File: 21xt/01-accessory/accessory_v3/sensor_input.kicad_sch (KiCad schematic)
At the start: 3 parts, among them J1 Conn_02x23_Counter_Clockwise, J2 Mezzanine Edge

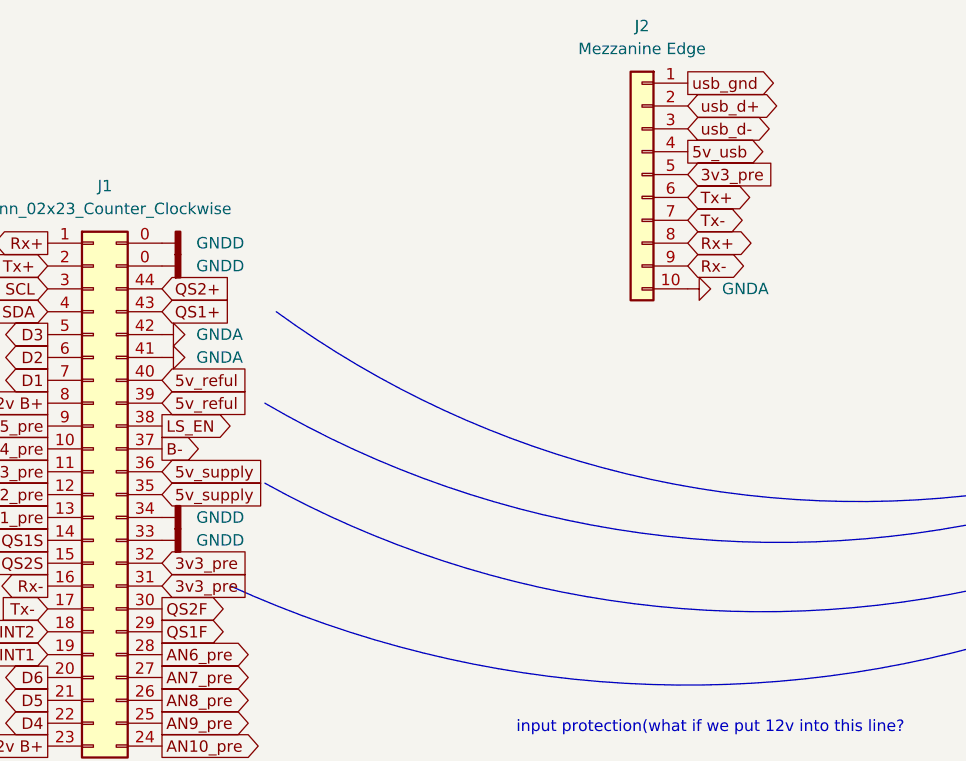
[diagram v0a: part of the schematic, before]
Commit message: prod
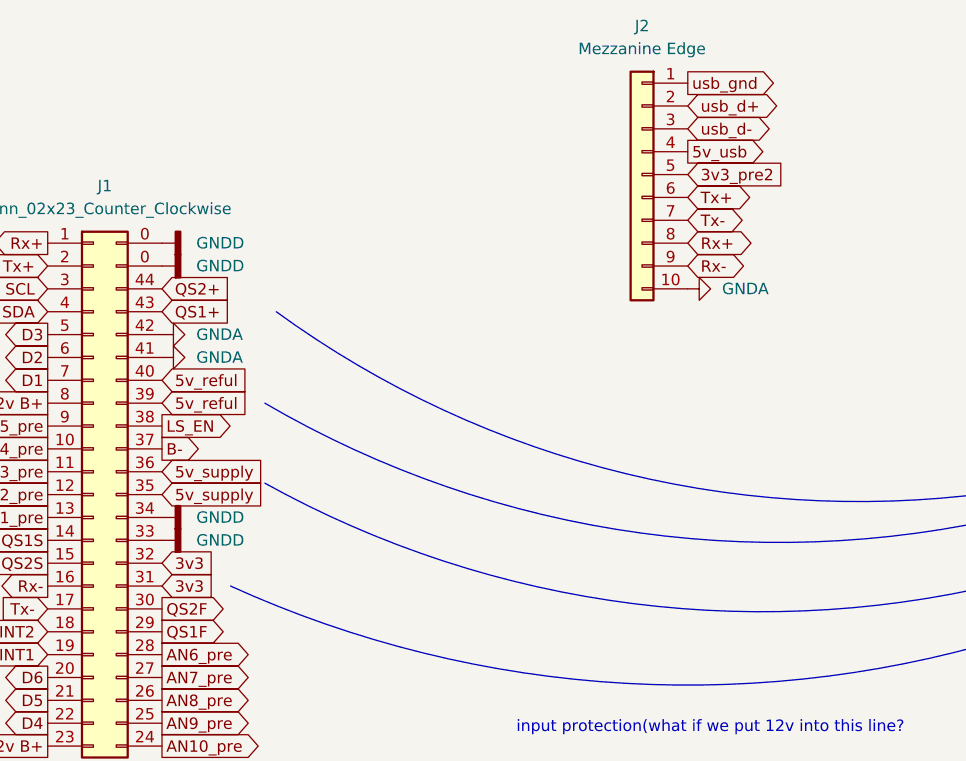
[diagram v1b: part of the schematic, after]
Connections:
- net 3v3_pre renamed 3v3
- net 3v3: no longer J2.5 (Pin_5)
- new net 3v3_pre2: J2.5 (Pin_5)
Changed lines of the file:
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@@
+		)
+	)
+	(global_label "3v3"
+		(shape input)
+		(at 139.7 102.87 0)
+		(fields_autoplaced yes)
+		(effects
+			(font
+				(size 1.27 1.27)
+			)
+			(justify left)
+		)
+		(property "Intersheetrefs" "${INTERSHEET_REFS}"
+			(at 146.0718 102.87 0)
+			(effects
+				(font
+					(size 1.27 1.27)
+				)
+				(justify left)
+				(hide yes)
+			)
 		)
 	)
@@
 		)
 	)
-	(global_label "3v3_pre"
-		(shape input)
-		(at 139.7 102.87 0)
-		(fields_autoplaced yes)
-		(effects
-			(font
-				(size 1.27 1.27)
-			)
-			(justify left)
-		)
-		(property "Intersheetrefs" "${INTERSHEET_REFS}"
-			(at 150.0632 102.87 0)
-			(effects
-				(font
-					(size 1.27 1.27)
-				)
-				(justify left)
-				(hide yes)
-			)
-		)
-	)
 	(global_label "12v B+"
 		(shape output)
@@
 		)
 	)
+	(global_label "3v3_pre2"
+		(shape input)
+		(at 198.12 59.69 0)
+		(fields_autoplaced yes)
+		(effects
+			(font
+				(size 1.27 1.27)
+			)
+			(justify left)
+		)
+		(property "Intersheetrefs" "${INTERSHEET_REFS}"
+			(at 209.6927 59.69 0)
+			(effects
+				(font
+					(size 1.27 1.27)
+				)
+				(justify left)
+				(hide yes)
+			)
+		)
+	)
 	(global_label "GPIO{slash}INT2"
 		(shape bidirectional)
@@
 		)
 	)
+	(global_label "3v3"
+		(shape input)
+		(at 139.7 105.41 0)
+		(fields_autoplaced yes)
+		(effects
+			(font
+				(size 1.27 1.27)
+			)
+			(justify left)
+		)
+		(property "Intersheetrefs" "${INTERSHEET_REFS}"
+			(at 146.0718 105.41 0)
+			(effects
+				(font
+					(size 1.27 1.27)
+				)
+				(justify left)
+				(hide yes)
+			)
+		)
+	)
 	(global_label "AN7_pre"
 		(shape output)
@@
 		)
 	)
-	(global_label "3v3_pre"
-		(shape input)
-		(at 139.7 105.41 0)
-		(fields_autoplaced yes)
-		(effects
-			(font
-				(size 1.27 1.27)
-			)
-			(justify left)
-		)
-		(property "Intersheetrefs" "${INTERSHEET_REFS}"
-			(at 150.0632 105.41 0)
-			(effects
-				(font
-					(size 1.27 1.27)
-				)
-				(justify left)
-				(hide yes)
-			)
-		)
-	)
 	(global_label "Tx-"
 		(shape input)
@@
 			(effects
 				(font
-					(size 1.27 1.27)
-				)
-				(justify left)
-				(hide yes)
-			)
-		)
-	)
-	(global_label "3v3_pre"
-		(shape input)
-		(at 198.12 59.69 0)
-		(fields_autoplaced yes)
-		(effects
-			(font
-				(size 1.27 1.27)
-			)
-			(justify left)
-		)
-		(property "Intersheetrefs" "${INTERSHEET_REFS}"
-			(at 208.4832 59.69 0)
-			(effects
-				(font
